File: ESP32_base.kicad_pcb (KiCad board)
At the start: 4 copper layers, 112 x 54.9 mm, 40 parts, among them J1 Conn_01x16_Socket, J2 Conn_01x16_Socket, J5 KH-IPEXA-SMAKWE-B080H, SW1 boot, SW2 reset, U1 ADT7310TRZ, U2 3.3V, U3 ESP32-C5-WROOM-1U-N8-R8, U4 MCP23017-E/SO

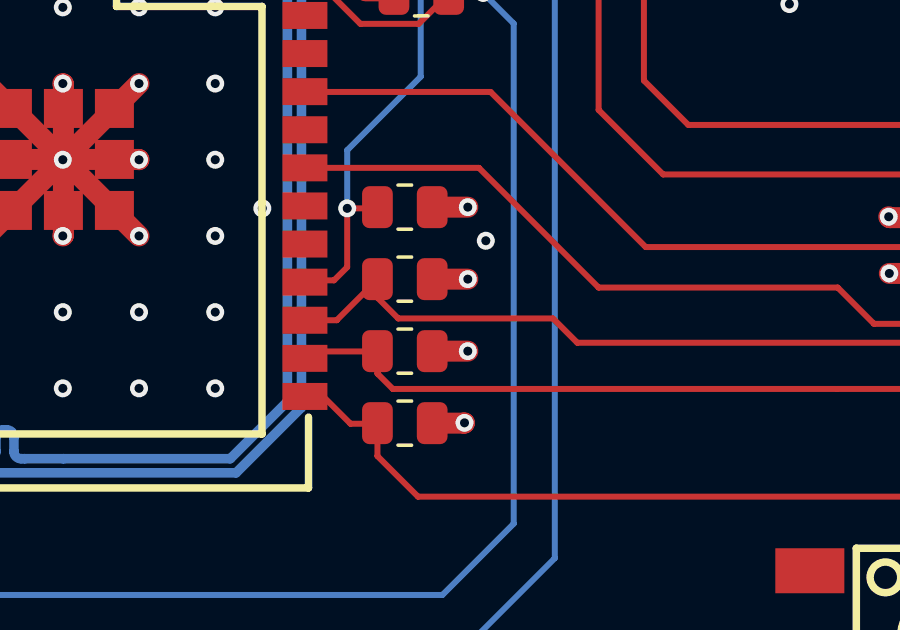
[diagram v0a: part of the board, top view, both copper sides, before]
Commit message: wip
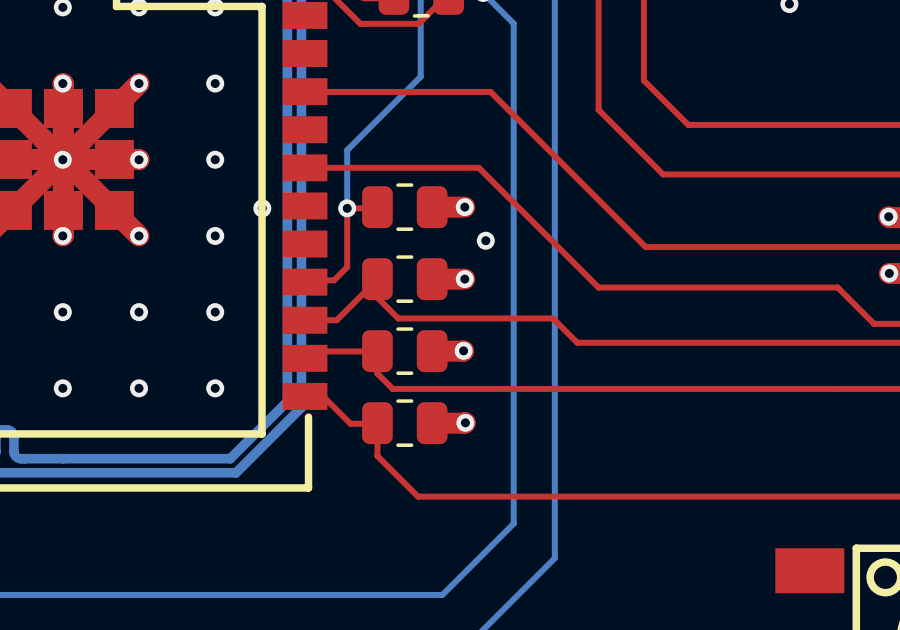
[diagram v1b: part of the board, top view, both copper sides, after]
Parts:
- C4: value C -> 10uF
- U2: value 3.3V -> AP63203WU-7
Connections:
- USBC1 pad 1: (no net) -> GND
- USBC1 pad 2: (no net) -> GND
- USBC1 pad 3: (no net) -> GND
- USBC1 pad 4: (no net) -> GND
